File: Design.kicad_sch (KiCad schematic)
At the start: 8 parts, among them U1 TP4056

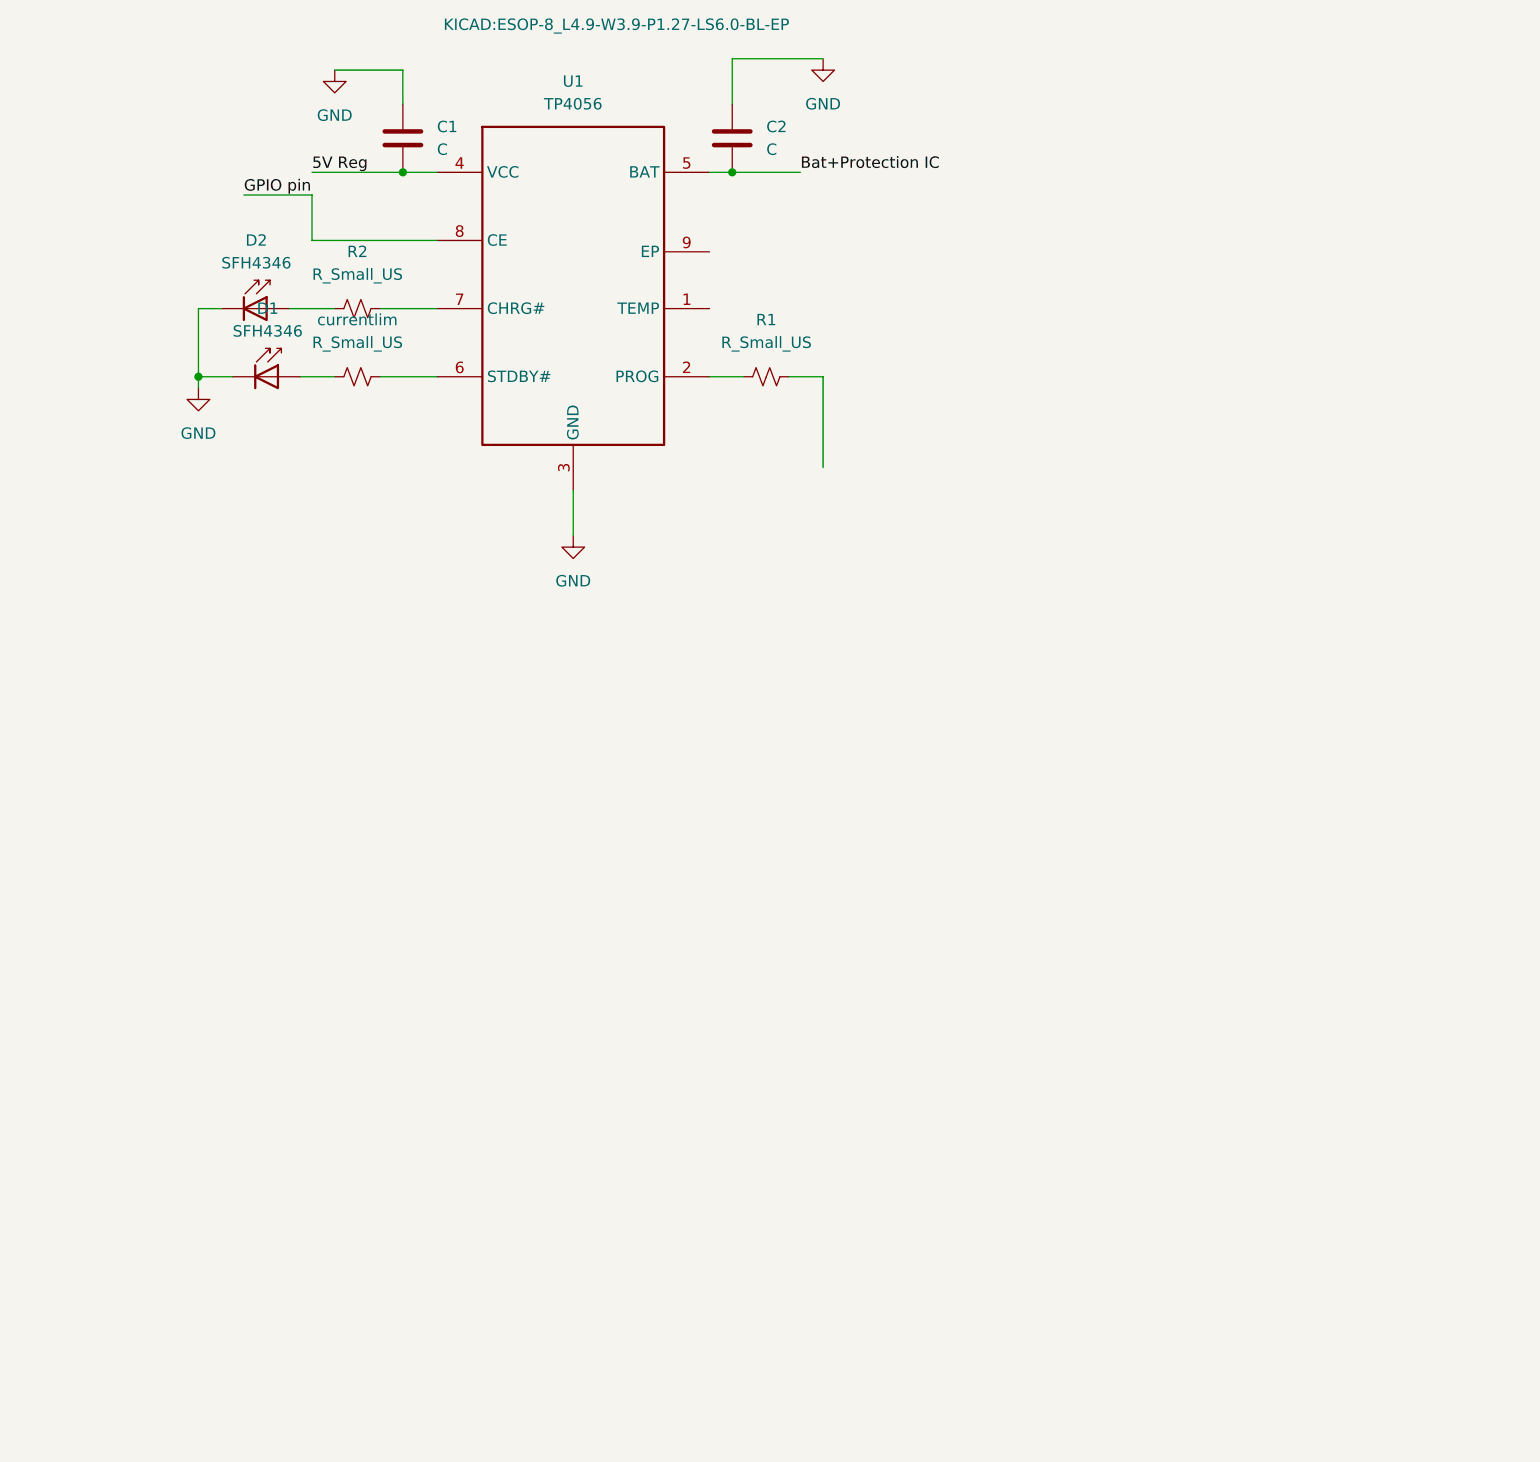
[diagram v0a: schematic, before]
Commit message: Add files via upload
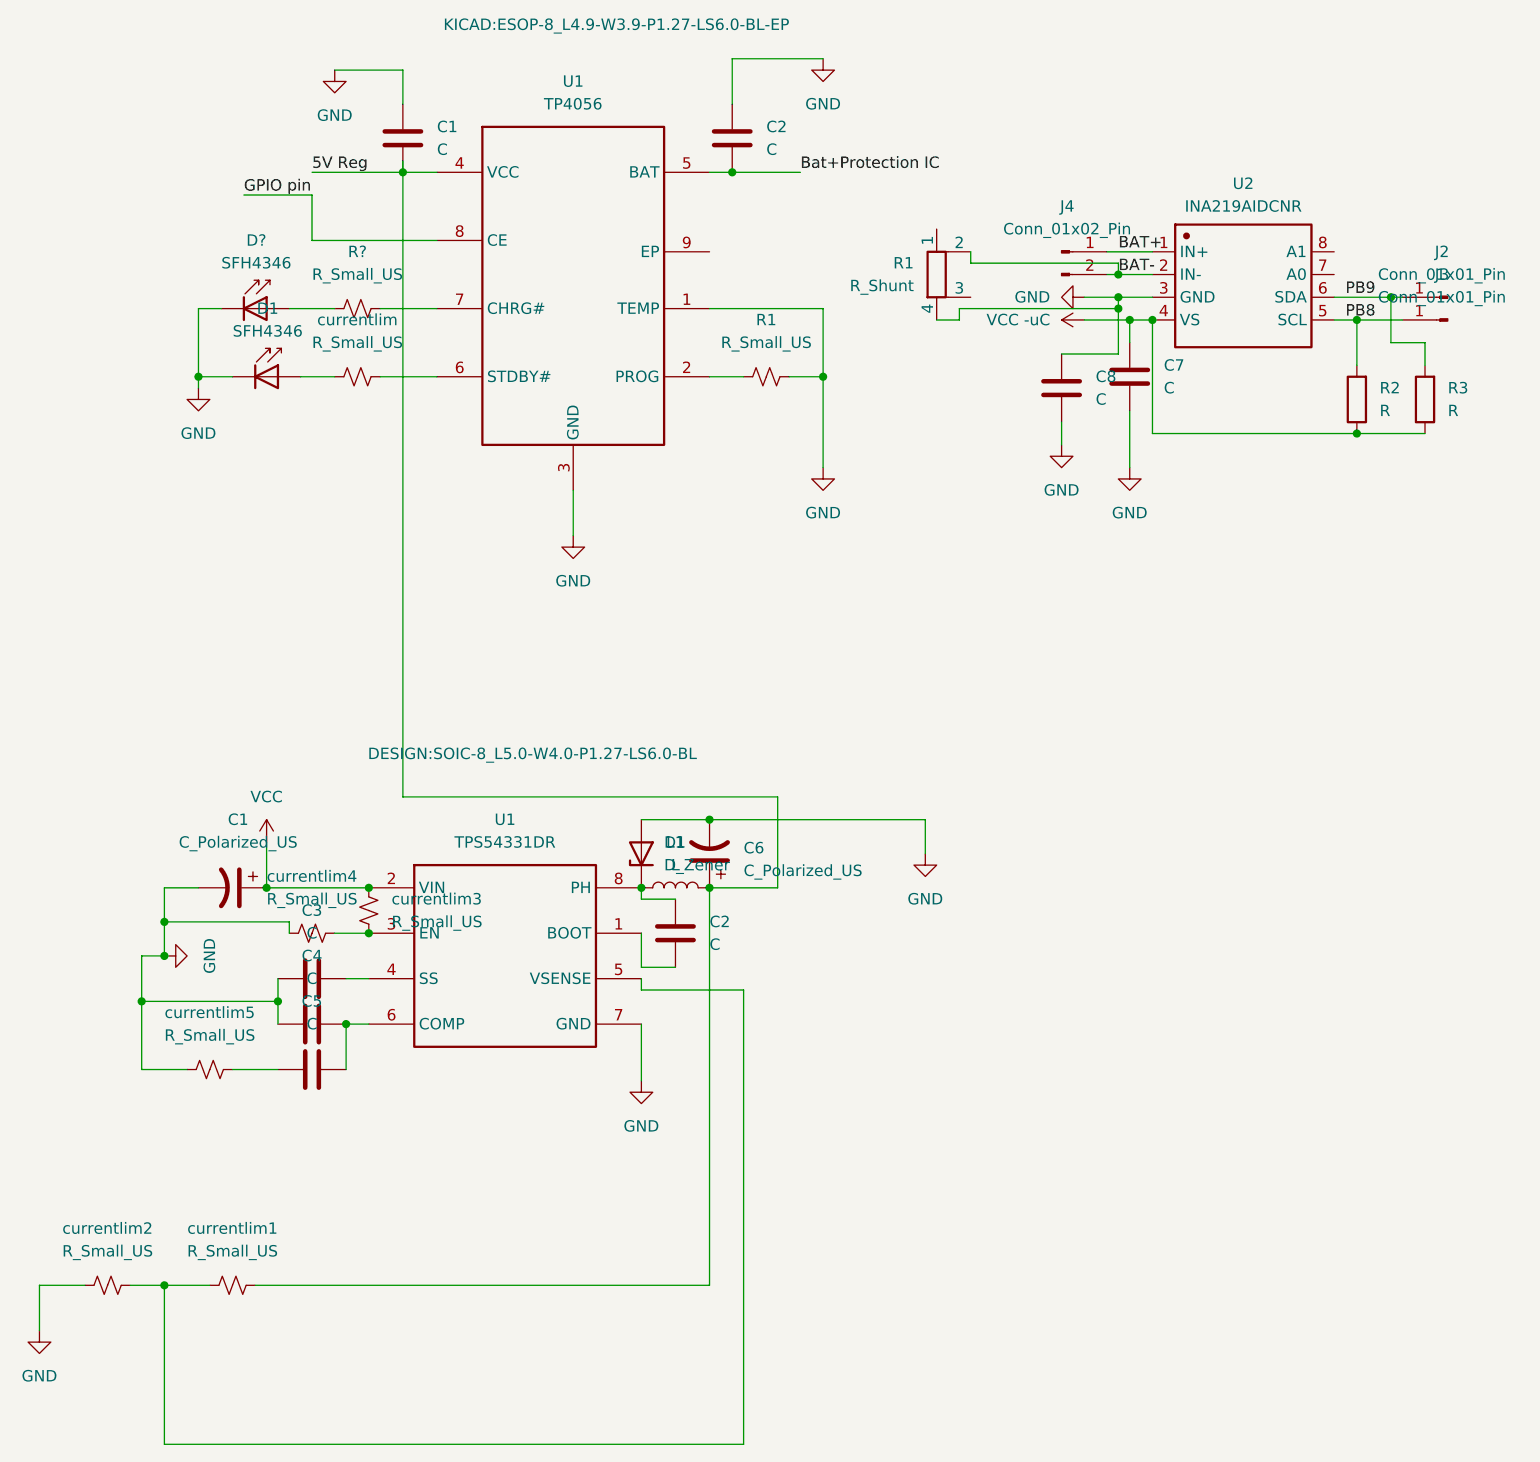
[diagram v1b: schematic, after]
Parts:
- added C1, C6: C_Polarized_US, symbol Device:C_Polarized_US
- added C2, C3, C4, C5, C7, C8: C, symbol Device:C
- added D1: D_Zener, symbol Device:D_Zener
- added J2, J3: Conn_01x01_Pin, symbol Connector:Conn_01x01_Pin
- added J4: Conn_01x02_Pin, symbol Connector:Conn_01x02_Pin
- added L1: L, symbol Device:L
- added R1: R_Shunt, symbol Device:R_Shunt
- added R2, R3: R, symbol Device:R
- added U1: TPS54331DR, DESIGN:SOIC-8_L5.0-W4.0-P1.27-LS6.0-BL, symbol SCHLIB_TPS54331DR_2025-03-24:TPS54331DR
- added U2: INA219AIDCNR, symbol SCHLIB_INA219AIDCNR_2025-03-24:INA219AIDCNR
- added currentlim1, currentlim2, currentlim3, currentlim4, currentlim5: R_Small_US, symbol Device:R_Small_US
- renumbered D2 to D?, R2 to R?
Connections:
- net 5V Reg: now also C6.1, L1.2, currentlim1.1
- net GND: now also R1.2, U1.1 (TEMP), C1.2, C3.1, C4.1, C6.2, C7.2, C8.1, C8.2, D1.2 (A), R1.4, U1.7 (GND), U2.3 (GND), currentlim2.2, currentlim4.1, currentlim5.2
- new net: U1.5 (VSENSE), currentlim1.2, currentlim2.1
- new net: C5.1, currentlim5.1
- new net: C4.2, C5.2, U1.6 (COMP)
- new net: U1.3 (EN), currentlim3.2, currentlim4.2
- new net: C2.1, D1.1 (K), L1.1, U1.8 (PH)
- new net: C2.2, U1.1 (BOOT)
- new net: C3.2, U1.4 (SS)
- new net BAT+: J4.1 (Pin_1), U2.1 (IN+)
- new net BAT-: J4.2 (Pin_2), R1.2, U2.2 (IN-)
- new net PB8: J3.1 (Pin_1), R2.2, U2.5 (SCL)
- new net PB9: J2.1 (Pin_1), R3.2, U2.6 (SDA)
- new net VCC: C1.1, U1.2 (VIN), currentlim3.1
- new net VCC -uC: C7.1, R2.1, R3.1, U2.4 (VS)
